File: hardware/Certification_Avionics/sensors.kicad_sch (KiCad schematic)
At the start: 24 parts, among them J6 MicroSDReader, J7 Conn_01x20_Pin, J8 Conn_01x20_Pin, Q1 NMOS, SW3 SW_DIP_x01, U6 BNO055, U7 BMP388

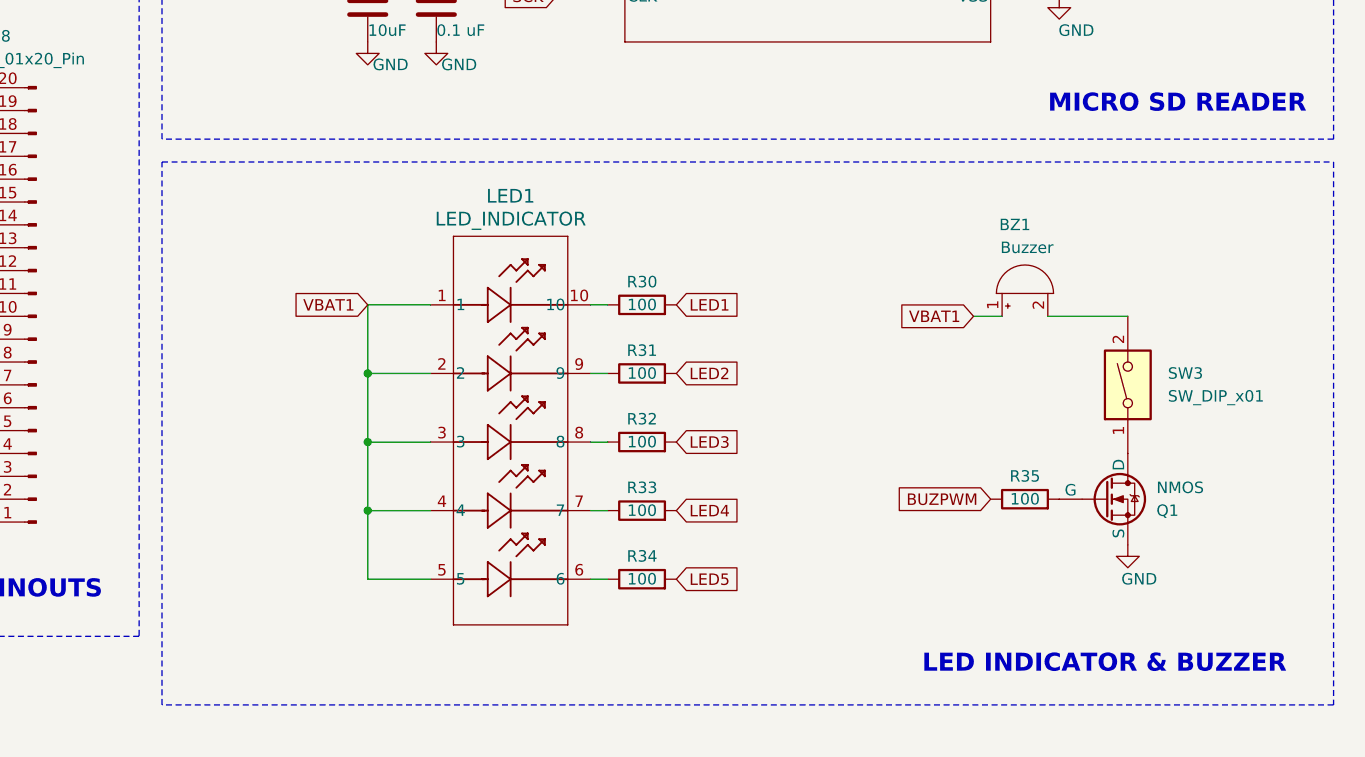
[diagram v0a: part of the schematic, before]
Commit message: Add comments to cert avionics
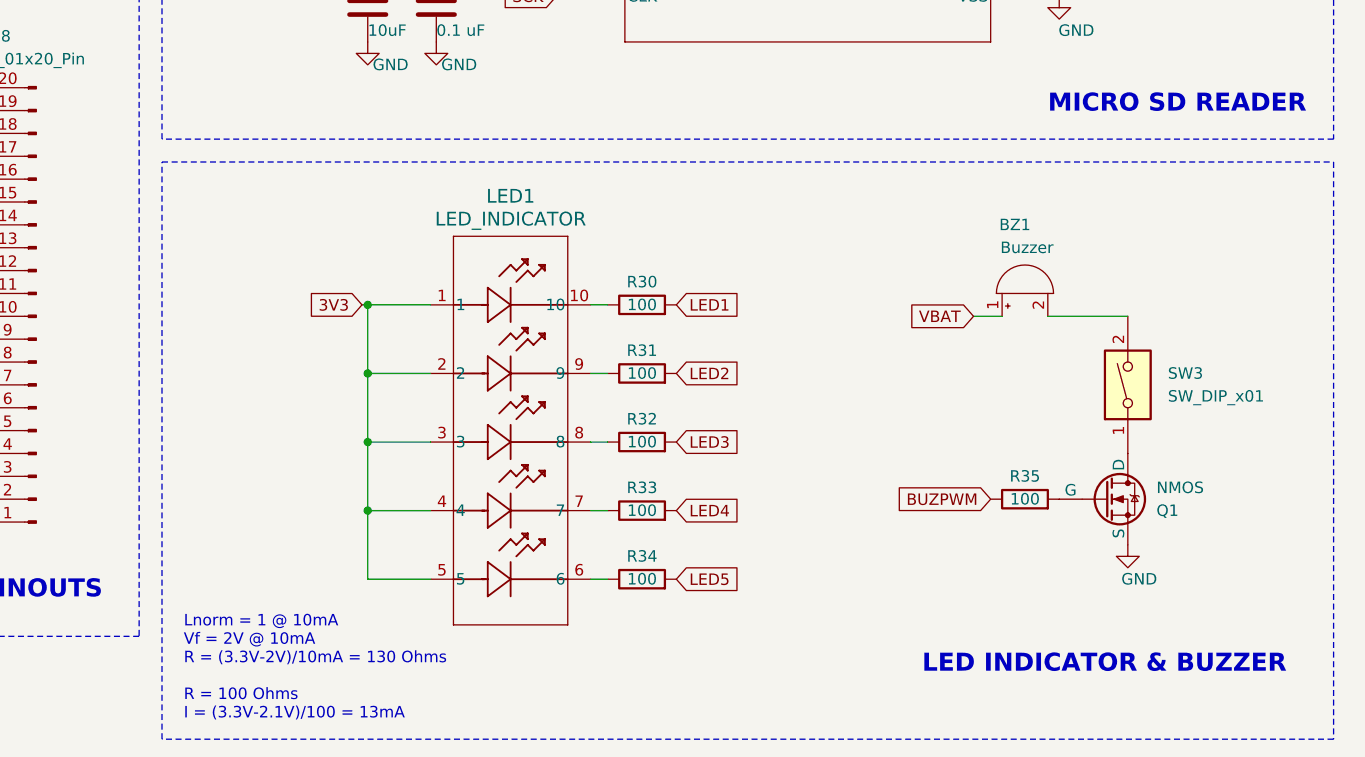
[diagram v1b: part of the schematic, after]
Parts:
- U6: Alternative (none) -> https://mm.digikey.com/Volume0/opasdata/d220001/medias/docu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
- U7: Alternative (none) -> https://www.bosch-sensortec.com/media/boschsensortec/downlo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
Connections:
- net 3V3: now also LED1.1, LED1.2, LED1.3, LED1.4, LED1.5
- removed net VBAT1: BZ1.1 (-), LED1.1, LED1.2, LED1.3, LED1.4, LED1.5
- new net VBAT: BZ1.1 (-)
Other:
- note added: "Lnorm = 1 @ 10mA Vf = 2V @ 10mA R = (3.3V-2V)/10mA = 130 Ohms R = 100 Ohms I = (3.3V-2.1V)/100 = 13mA"
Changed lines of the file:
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@@
 	)
 	(junction
+		(at 174.625 115.57)
+		(diameter 0)
+		(color 0 0 0 0)
+	)
+	(junction
 		(at 174.625 130.81)
 		(diameter 0)
@@
 	(wire
 		(pts
-			(xy 181.61 115.57) (xy 174.625 115.57)
-		)
-		(stroke
-			(width 0)
-			(type default)
-		)
-	)
-	(wire
-		(pts
 			(xy 182.245 78.74) (xy 195.58 78.74)
 		)
@@
 	(wire
 		(pts
+			(xy 173.99 115.57) (xy 174.625 115.57)
+		)
+		(stroke
+			(width 0)
+			(type default)
+		)
+	)
+	(wire
+		(pts
 			(xy 201.295 31.115) (xy 201.295 28.575)
 		)
@@
 	(wire
 		(pts
+			(xy 174.625 115.57) (xy 181.61 115.57)
+		)
+		(stroke
+			(width 0)
+			(type default)
+		)
+	)
+	(wire
+		(pts
 			(xy 55.88 33.02) (xy 47.625 33.02)
 		)
@@
 	(rectangle
 		(start 151.765 99.695)
-		(end 281.94 160.02)
+		(end 281.94 163.83)
 		(stroke
 			(width 0)
@@
 		)
 	)
+	(text "Lnorm = 1 @ 10mA\nVf = 2V @ 10mA\nR = (3.3V-2V)/10mA = 130 Ohms\n\nR = 100 Ohms\nI = (3.3V-2.1V)/100 = 13mA"
+		(exclude_from_sim no)
+		(at 154.178 155.956 0)
+		(effects
+			(font
+				(size 1.27 1.27)
+			)
+			(justify left)
+		)
+	)
 	(global_label "PWM2"
 		(shape input)
@@
 		)
 	)
-	(global_label "VBAT1"
+	(global_label "VBAT"
 		(shape input)
 		(at 241.935 116.84 180)
@@
 		)
 		(property "Intersheetrefs" "${INTERSHEET_REFS}"
-			(at 233.3255 116.84 0)
+			(at 234.535 116.84 0)
 			(effects
 				(font
@@
 		)
 	)
-	(global_label "VBAT1"
-		(shape input)
-		(at 174.625 115.57 180)
-		(fields_autoplaced yes)
-		(effects
-			(font
-				(size 1.27 1.27)
-			)
-			(justify right)
-		)
-		(property "Intersheetrefs" "${INTERSHEET_REFS}"
-			(at 166.0155 115.57 0)
-			(effects
-				(font
-					(size 1.27 1.27)
-				)
-				(justify right)
-				(hide yes)
-			)
-		)
-	)
 	(global_label "SDA"
 		(shape input)
@@
 		)
 	)
+	(global_label "3V3"
+		(shape input)
+		(at 173.99 115.57 180)
+		(fields_autoplaced yes)
+		(effects
+			(font
+				(size 1.27 1.27)
+			)
+			(justify right)
+		)
+		(property "Intersheetrefs" "${INTERSHEET_REFS}"
+			(at 167.4972 115.57 0)
+			(effects
+				(font
+					(size 1.27 1.27)
+				)
+				(justify right)
+				(hide yes)
+			)
+		)
+	)
 	(global_label "LED2"
 		(shape input)
@@
 			)
 		)
-		(property "Datasheet" "https://ngspice.sourceforge.io/docs/ngspice-manual.pdf"
+		(property "Datasheet" "https://goodarksemi.com/docs/datasheets/mosfets/GSFC0500.pdf"
 			(at 256.54 149.86 0)
 			(effects
@@
 			)
 		)
-		(property "Datasheet" "XGUGX5D"
+		(property "Datasheet" "https://www.sunledusa.com/products/spec/XGUGX5D.pdf"
 			(at 181.61 115.57 0)
 			(effects
@@
 			)
 		)
-		(property "Datasheet" "~"
+		(property "Datasheet" "https://www.sameskydevices.com/product/resource/cpt-1404-85t.pdf"
 			(at 245.11 114.935 90)
 			(effects
@@
 			)
 		)
-		(property "Datasheet" "BNO055"
+		(property "Datasheet" "https://www.bosch-sensortec.com/media/boschsensortec/downloads/datasheets/bst-bno055-ds000.pdf"
 			(at 55.88 33.02 0)
 			(effects
@@
 			)
 		)
+		(property "Alternative" "https://mm.digikey.com/Volume0/opasdata/d220001/medias/docus/6531/BNO080_085_Datasheet-3196201.pdf"
+			(at 55.88 33.02 0)
+			(effects
+				(font
+					(size 1.27 1.27)
+				)
+				(hide yes)
+			)
+		)
 		(pin "1"
 		)
@@
 			)
 		)
-		(property "Datasheet" "BMP388"
+		(property "Datasheet" "https://www.bosch-sensortec.com/media/boschsensortec/downloads/datasheets/bst-bmp388-ds001.pdf"
 			(at 224.79 25.4 0)
 			(effects
@@
 			)
 		)
+		(property "Alternative" "https://www.bosch-sensortec.com/media/boschsensortec/downloads/datasheets/bst-bmp581-ds004.pdf"
+			(at 204.47 28.575 0)
+			(effects
+				(font
+					(size 1.27 1.27)
+				)
+				(hide yes)
+			)
+		)
 		(pin "1"
 		)
@@
 			)
 		)
-		(property "Datasheet" "1040310811"
+		(property "Datasheet" "https://www.molex.com/en-us/products/part-detail/1040310811?display=pdf"
 			(at 195.58 71.12 0)
 			(effects
